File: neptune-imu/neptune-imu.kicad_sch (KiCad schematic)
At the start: 4 parts, among them SW1 reset, U1 STM32L432KCUx

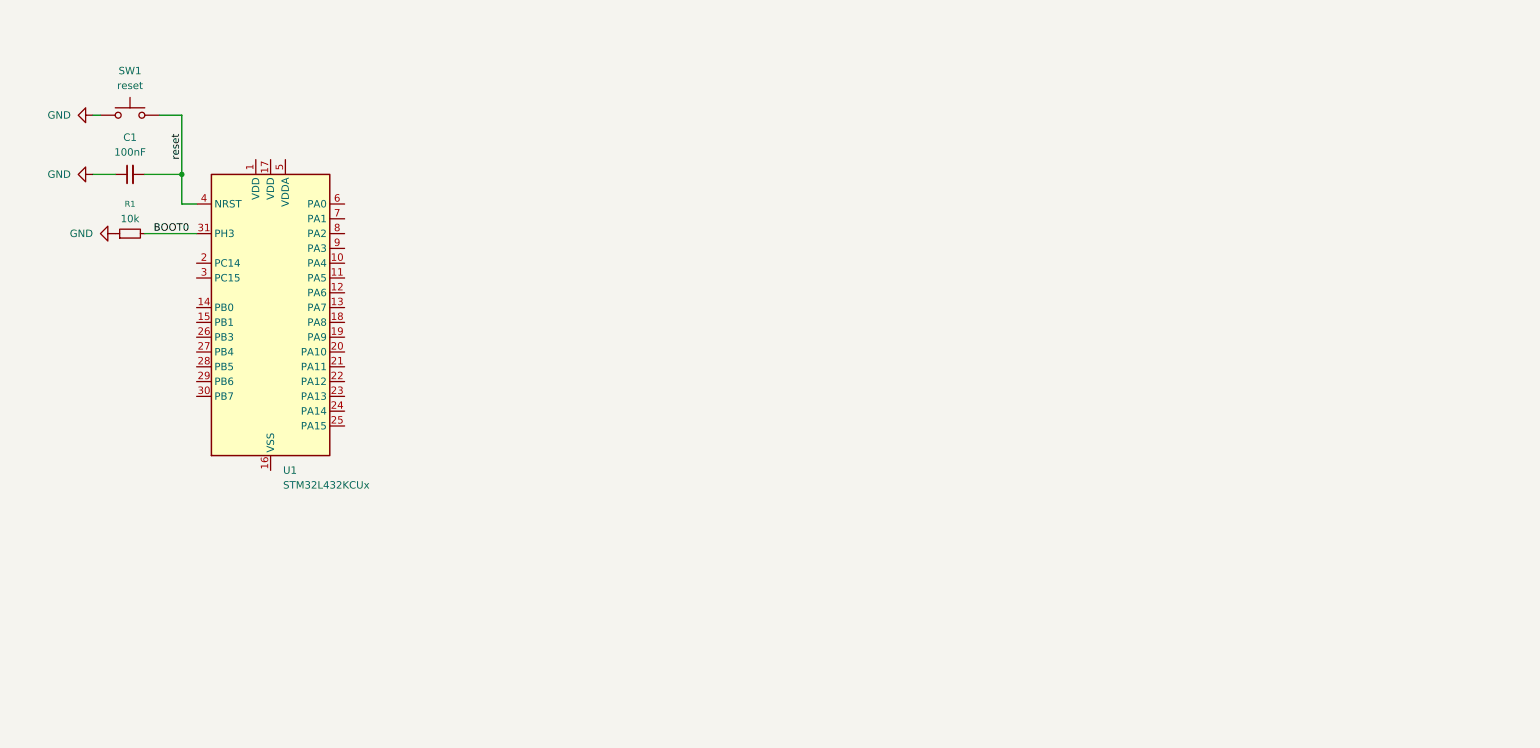
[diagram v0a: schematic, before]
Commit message: no summary
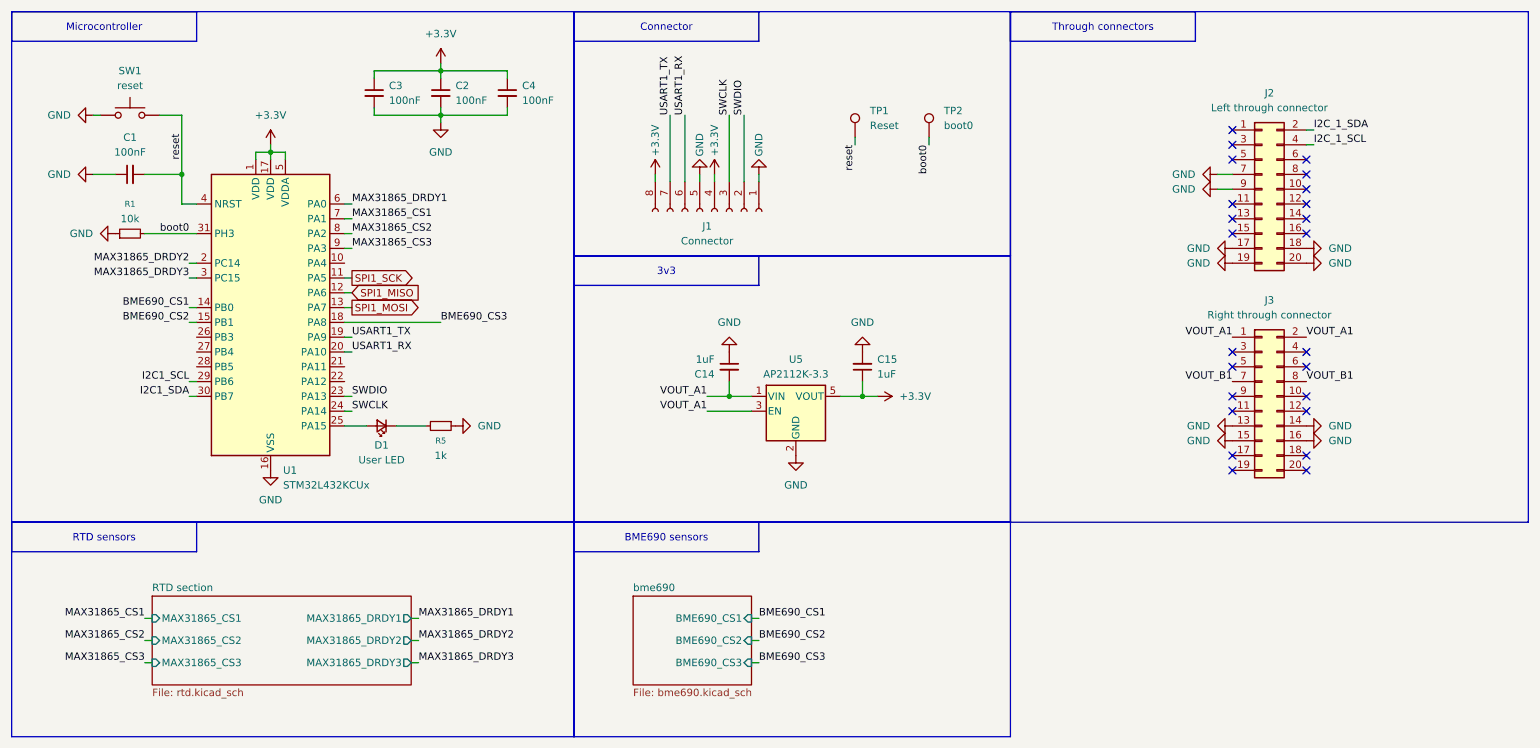
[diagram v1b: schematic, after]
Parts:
- added C14, C15: 1uF, Capacitor_SMD:C_0603_1608Metric, symbol Device:C_Small
- added C2, C3, C4: 100nF, Capacitor_SMD:C_0402_1005Metric, symbol Device:C_Small
- added D1: User LED, LED_SMD:LED_0603_1608Metric, symbol Device:LED_Small
- added J1: Connector, neptune-imu-footprints:HDR-SMD_8P-P2.00-H-F-W9.2, symbol Connector:Conn_01x08_Socket
- added J2: Left through connector, neptune-imu-footprints:gaia_connector, symbol Connector_Generic:Conn_02x10_Odd_Even
- added J3: Right through connector, neptune-imu-footprints:gaia_connector, symbol Connector_Generic:Conn_02x10_Odd_Even
- added R5: 1k, Resistor_SMD:R_0402_1005Metric, symbol Device:R_Small
- added TP1: Reset, TestPoint:TestPoint_Pad_2.0x2.0mm, symbol Connector:TestPoint
- added TP2: boot0, TestPoint:TestPoint_Pad_2.0x2.0mm, symbol Connector:TestPoint
- added U5: AP2112K-3.3, Package_TO_SOT_SMD:SOT-23-5, symbol Regulator_Linear:AP2112K-3.3
- C1: footprint (none) -> Capacitor_SMD:C_0402_1005Metric
- R1: footprint (none) -> Resistor_SMD:R_0402_1005Metric
- SW1: footprint (none) -> neptune-imu-footprints:KEY-SMD_L4.0-W3.0-LS4.9-1
- U1: footprint Package_DFN_QFN:QFN-32-1EP_5x5mm_P0.5mm_EP3.45x3.45mm -> neptune-imu-footprints:STM32L432KCUx
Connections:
- net GND: now also U1.16 (VSS), U1.32 (VSS), U1.33 (VSS), C14.1, C15.2, C2.2, C3.2, C4.2, J1.1 (Pin_1), J1.5 (Pin_5), J2.17 (Pin_17), J2.18 (Pin_18), J2.19 (Pin_19), J2.20 (Pin_20), J2.7 (Pin_7), J2.9 (Pin_9), J3.13 (Pin_13), J3.14 (Pin_14), J3.15 (Pin_15), J3.16 (Pin_16), R5.1, U5.2 (GND)
- net reset: now also TP1.1
- net +3.3V: now reaches U1.1 (VDD)
- net +3.3V: now also U1.17 (VDD), U1.5 (VDDA), C15.1, C2.1, C3.1, C4.1, J1.4 (Pin_4), J1.8 (Pin_8), U5.5 (VOUT)
- net SPI1_SCK: now reaches U1.11 (PA5)
- net SPI1_MISO: now reaches U1.12 (PA6)
- net SPI1_MOSI: now reaches U1.13 (PA7)
- net BME690_CS1: now reaches U1.14 (PB0)
- net BME690_CS2: now reaches U1.15 (PB1)
- net BME690_CS3: now reaches U1.18 (PA8)
- net USART1_TX: now reaches U1.19 (PA9)
- net USART1_TX: now also J1.7 (Pin_7)
- net MAX31865_DRDY2: now reaches U1.2 (PC14)
- net USART1_RX: now reaches U1.20 (PA10)
- net USART1_RX: now also J1.6 (Pin_6)
- net SWDIO: now reaches U1.23 (PA13)
- net SWDIO: now also J1.2 (Pin_2)
- net SWCLK: now reaches U1.24 (PA14)
- net SWCLK: now also J1.3 (Pin_3)
- net at U1.25 (PA15): now also D1.2 (A)
- net I2C1_SCL: now reaches U1.29 (PB6)
- net MAX31865_DRDY3: now reaches U1.3 (PC15)
- net I2C1_SDA: now reaches U1.30 (PB7)
- net MAX31865_DRDY1: now reaches U1.6 (PA0)
- net MAX31865_CS1: now reaches U1.7 (PA1)
- net MAX31865_CS2: now reaches U1.8 (PA2)
- net MAX31865_CS3: now reaches U1.9 (PA3)
- net BOOT0 renamed boot0
- net boot0: now also TP2.1
- new net: D1.1 (K), R5.2
- new net I2C_1_SCL: J2.4 (Pin_4)
- new net I2C_1_SDA: J2.2 (Pin_2)
- new net VOUT_A1: C14.2, J3.1 (Pin_1), J3.2 (Pin_2), U5.1 (VIN), U5.3 (EN)
- new net VOUT_B1: J3.7 (Pin_7), J3.8 (Pin_8)
- no-connect marks 0 -> 24
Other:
- added sheet RTD section (rtd.kicad_sch)
- added sheet bme690 (bme690.kicad_sch)
- title: IMU PCB -> ENV PCB
